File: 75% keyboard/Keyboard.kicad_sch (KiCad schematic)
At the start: 166 parts, among them SW1 RotaryEncoder, U1 nice_nano

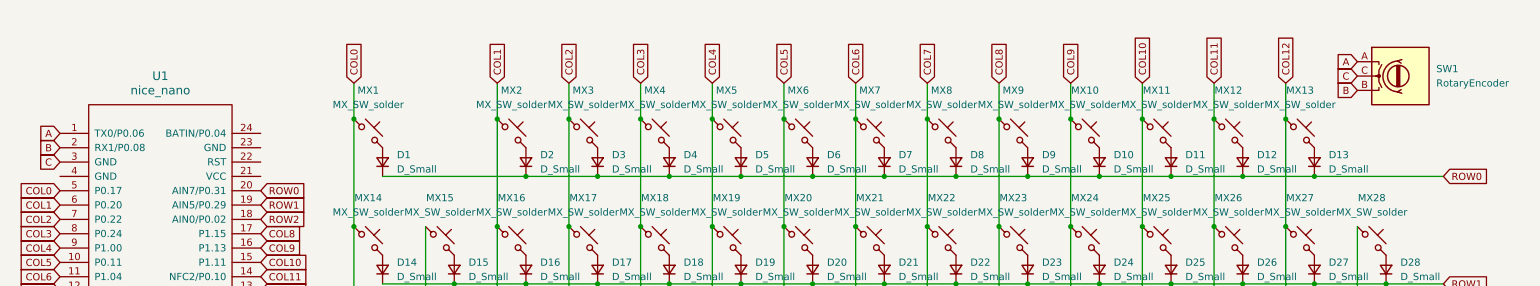
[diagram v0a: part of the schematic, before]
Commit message: kicad files
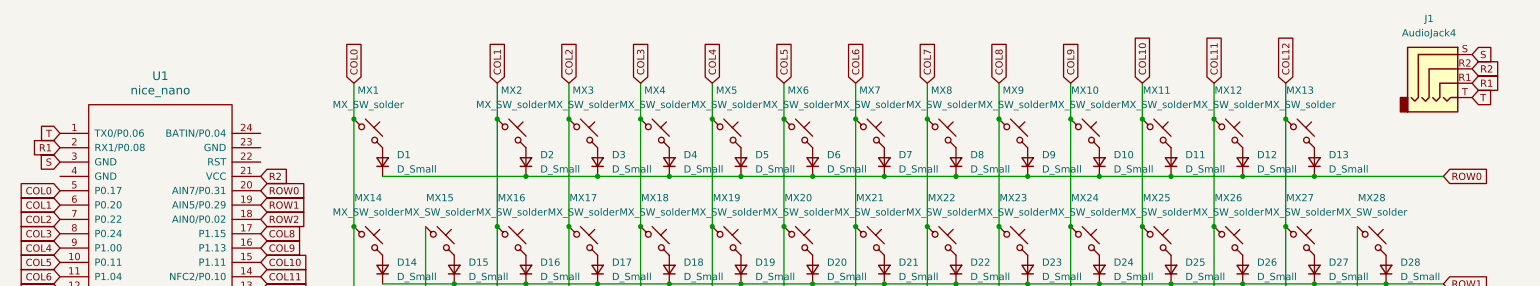
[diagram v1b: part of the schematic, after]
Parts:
- removed SW1: RotaryEncoder, Rotary Encoder:Bourns-PEC11R-4220F-S0024-0-0-0, symbol Device:RotaryEncoder
- added J1: AudioJack4, Connector_Audio:Jack_3.5mm_PJ320D_Horizontal, symbol Connector_Audio:AudioJack4
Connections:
- net R2: now reaches U1.21 (VCC)
- net R2: now also J1.R2
- net A renamed T
- net T: now also J1.T
- net B renamed R1
- net R1: now also J1.R1
- net C renamed S
- net S: now also J1.S
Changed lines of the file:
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@@
 		)
 	)
+	(global_label "R2"
+		(shape input)
+		(at 58.42 52.07 0)
+		(fields_autoplaced yes)
+		(effects
+			(font
+				(size 1.27 1.27)
+			)
+			(justify left)
+		)
+		(property "Intersheetrefs" "${INTERSHEET_REFS}"
+			(at 63.8847 52.07 0)
+			(effects
+				(font
+					(size 1.27 1.27)
+				)
+				(justify left)
+				(hide yes)
+			)
+		)
+	)
 	(global_label "COL4"
 		(shape input)
@@
 		)
 	)
-	(global_label "A"
-		(shape input)
-		(at 22.86 44.45 180)
-		(fields_autoplaced yes)
-		(effects
-			(font
-				(size 1.27 1.27)
-			)
-			(justify right)
-		)
-		(property "Intersheetrefs" "${INTERSHEET_REFS}"
-			(at 18.7862 44.45 0)
-			(effects
-				(font
-					(size 1.27 1.27)
-				)
-				(justify right)
-				(hide yes)
-			)
-		)
-	)
-	(global_label "B"
-		(shape input)
-		(at 252.73 36.83 180)
-		(fields_autoplaced yes)
-		(effects
-			(font
-				(size 1.27 1.27)
-			)
-			(justify right)
-		)
-		(property "Intersheetrefs" "${INTERSHEET_REFS}"
-			(at 248.4748 36.83 0)
-			(effects
-				(font
-					(size 1.27 1.27)
-				)
-				(justify right)
-				(hide yes)
-			)
-		)
-	)
 	(global_label "COL1"
 		(shape input)
@@
 		)
 	)
-	(global_label "C"
+	(global_label "COL12"
 		(shape input)
-		(at 22.86 49.53 180)
+		(at 58.42 72.39 0)
 		(fields_autoplaced yes)
 		(effects
@@
 				(size 1.27 1.27)
 			)
-			(justify right)
+			(justify left)
 		)
 		(property "Intersheetrefs" "${INTERSHEET_REFS}"
-			(at 18.6048 49.53 0)
+			(at 67.4528 72.39 0)
 			(effects
 				(font
 					(size 1.27 1.27)
 				)
-				(justify right)
+				(justify left)
 				(hide yes)
 			)
 		)
 	)
-	(global_label "COL12"
+	(global_label "ROW2"
 		(shape input)
-		(at 58.42 72.39 0)
+		(at 58.42 59.69 0)
 		(fields_autoplaced yes)
 		(effects
@@
 		)
 		(property "Intersheetrefs" "${INTERSHEET_REFS}"
-			(at 67.4528 72.39 0)
+			(at 66.6666 59.69 0)
 			(effects
 				(font
@@
 		)
 	)
-	(global_label "ROW2"
+	(global_label "S"
 		(shape input)
-		(at 58.42 59.69 0)
+		(at 273.05 30.48 0)
 		(fields_autoplaced yes)
 		(effects
@@
 		)
 		(property "Intersheetrefs" "${INTERSHEET_REFS}"
-			(at 66.6666 59.69 0)
+			(at 277.2447 30.48 0)
 			(effects
 				(font
@@
 		)
 	)
-	(global_label "B"
+	(global_label "T"
 		(shape input)
-		(at 22.86 46.99 180)
+		(at 273.05 38.1 0)
 		(fields_autoplaced yes)
 		(effects
@@
 				(size 1.27 1.27)
 			)
-			(justify right)
+			(justify left)
 		)
 		(property "Intersheetrefs" "${INTERSHEET_REFS}"
-			(at 18.6048 46.99 0)
+			(at 277.0028 38.1 0)
 			(effects
 				(font
 					(size 1.27 1.27)
 				)
-				(justify right)
+				(justify left)
 				(hide yes)
 			)
@@
 		)
 	)
+	(global_label "R1"
+		(shape input)
+		(at 22.86 46.99 180)
+		(fields_autoplaced yes)
+		(effects
+			(font
+				(size 1.27 1.27)
+			)
+			(justify right)
+		)
+		(property "Intersheetrefs" "${INTERSHEET_REFS}"
+			(at 17.3953 46.99 0)
+			(effects
+				(font
+					(size 1.27 1.27)
+				)
+				(justify right)
+				(hide yes)
+			)
+		)
+	)
 	(global_label "COL8"
 		(shape input)
@@
 		)
 	)
+	(global_label "S"
+		(shape input)
+		(at 22.86 49.53 180)
+		(fields_autoplaced yes)
+		(effects
+			(font
+				(size 1.27 1.27)
+			)
+			(justify right)
+		)
+		(property "Intersheetrefs" "${INTERSHEET_REFS}"
+			(at 18.6653 49.53 0)
+			(effects
+				(font
+					(size 1.27 1.27)
+				)
+				(justify right)
+				(hide yes)
+			)
+		)
+	)
 	(global_label "COL12"
 		(shape input)
@@
 		)
 	)
-	(global_label "C"
+	(global_label "R2"
 		(shape input)
-		(at 252.73 34.29 180)
+		(at 273.05 33.02 0)
 		(fields_autoplaced yes)
 		(effects
@@
 				(size 1.27 1.27)
 			)
-			(justify right)
+			(justify left)
 		)
 		(property "Intersheetrefs" "${INTERSHEET_REFS}"
-			(at 248.4748 34.29 0)
+			(at 278.5147 33.02 0)
 			(effects
 				(font
 					(size 1.27 1.27)
 				)
-				(justify right)
+				(justify left)
 				(hide yes)
 			)
 		)
 	)
-	(global_label "COL2"
+	(global_label "R1"
 		(shape input)
-		(at 113.03 35.56 90)
+		(at 273.05 35.56 0)
 		(fields_autoplaced yes)
 		(effects
@@
 		)
 		(property "Intersheetrefs" "${INTERSHEET_REFS}"
-			(at 113.03 27.7367 90)
+			(at 278.5147 35.56 0)
 			(effects
 				(font
@@
 		)
 	)
-	(global_label "COL4"
+	(global_label "T"
 		(shape input)
-		(at 138.43 35.56 90)
+		(at 22.86 44.45 180)
+		(fields_autoplaced yes)
+		(effects
+			(font
+				(size 1.27 1.27)
+			)
+			(justify right)
+		)
+		(property "Intersheetrefs" "${INTERSHEET_REFS}"
+			(at 18.9072 44.45 0)
+			(effects
+				(font
+					(size 1.27 1.27)
+				)
+				(justify right)
+				(hide yes)
+			)
+		)
+	)
+	(global_label "COL2"
+		(shape input)
+		(at 113.03 35.56 90)
 		(fields_autoplaced yes)
 		(effects
@@
 		)
 		(property "Intersheetrefs" "${INTERSHEET_REFS}"
-			(at 138.43 27.7367 90)
+			(at 113.03 27.7367 90)
 			(effects
 				(font
@@
 		)
 	)
-	(global_label "A"
+	(global_label "COL4"
 		(shape input)
-		(at 252.73 31.75 180)
+		(at 138.43 35.56 90)
 		(fields_autoplaced yes)
 		(effects
@@
 				(size 1.27 1.27)
 			)
-			(justify right)
+			(justify left)
 		)
 		(property "Intersheetrefs" "${INTERSHEET_REFS}"
-			(at 248.6562 31.75 0)
+			(at 138.43 27.7367 90)
 			(effects
 				(font
 					(size 1.27 1.27)
 				)
-				(justify right)
+				(justify left)
 				(hide yes)
 			)
@@
 	)
 	(symbol
+		(lib_id "Connector_Audio:AudioJack4")
+		(at 267.97 33.02 0)
+		(unit 1)
+		(exclude_from_sim no)
+		(in_bom yes)
+		(on_board yes)
+		(dnp no)
+		(fields_autoplaced yes)
+		(property "Reference" "J1"
+			(at 265.43 24.13 0)
+			(effects
+				(font
+					(size 1.27 1.27)
+				)
+			)
+		)
+		(property "Value" "AudioJack4"
+			(at 265.43 26.67 0)
+			(effects
+				(font
+					(size 1.27 1.27)
+				)
+			)
+		)
+		(property "Footprint" "Connector_Audio:Jack_3.5mm_PJ320D_Horizontal"
+			(at 267.97 33.02 0)
+			(effects
+				(font
+					(size 1.27 1.27)
+				)
+				(hide yes)
+			)
+		)
+		(property "Datasheet" "~"
+			(at 267.97 33.02 0)
+			(effects
+				(font
+					(size 1.27 1.27)
+				)
+				(hide yes)
+			)
+		)
+		(property "Description" "Audio Jack, 4 Poles (TRRS)"
+			(at 267.97 33.02 0)
+			(effects
+				(font
+					(size 1.27 1.27)
+				)
+				(hide yes)
+			)
+		)
+		(pin "R1"
+		)
+		(pin "R2"
+		)
+		(pin "S"
+		)
+		(pin "T"
+		)
+		(instances
+			(project ""
+				(path "/565ab7be-6155-4b88-aa2d-6bfc06a6601a"
+					(reference "J1")
+					(unit 1)
+				)
+			)
+		)
+	)
+	(symbol
 		(lib_id "Device:D_Small")
 		(at 143.51 107.95 90)
@@
 					(unit 1)
 				)
-			)
-		)
-	)
-	(symbol
-		(lib_id "Device:RotaryEncoder")
-		(at 260.35 34.29 0)
-		(unit 1)
-		(exclude_from_sim no)
-		(in_bom yes)
-		(on_board yes)
-		(dnp no)
-		(fields_autoplaced yes)
-		(property "Reference" "SW1"
-			(at 266.7 33.0199 0)
-			(effects
-				(font
-					(size 1.27 1.27)
-				)
-				(justify left)
-			)
-		)
-		(property "Value" "RotaryEncoder"
-			(at 266.7 35.5599 0)
-			(effects
-				(font
-					(size 1.27 1.27)
-				)
-				(justify left)
-			)
-		)
-		(property "Footprint" "Rotary Encoder:Bourns-PEC11R-4220F-S0024-0-0-0"
-			(at 256.54 30.226 0)
-			(effects
-				(font
-					(size 1.27 1.27)
-				)
-				(hide yes)
-			)
-		)
-		(property "Datasheet" "~"
-			(at 260.35 27.686 0)
-			(effects
-				(font
-					(size 1.27 1.27)
-				)
-				(hide yes)
-			)
-		)
-		(property "Description" "Rotary encoder, dual channel, incremental quadrate outputs"
-			(at 260.35 34.29 0)
-			(effects
-				(font
-					(size 1.27 1.27)
-				)
-				(hide yes)
-			)
-		)
-		(pin "B"
-		)
-		(pin "A"
-		)
-		(pin "C"
-		)
-		(instances
-			(project ""
-				(path "/565ab7be-6155-4b88-aa2d-6bfc06a6601a"
-					(reference "SW1")
-					(unit 1)
-				)
